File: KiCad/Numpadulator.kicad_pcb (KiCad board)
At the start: 2 copper layers, 3.4 x 3 mm, 58 parts, among them SW1 Cherry_MX_RGB_WS2812, SW10 Cherry_MX_RGB_WS2812, SW11 Cherry_MX_RGB_WS2812, SW12 Cherry_MX_RGB_WS2812, SW13 Cherry_MX_RGB_WS2812, SW14 Cherry_MX_RGB_WS2812, SW15 Cherry_MX_RGB_WS2812, SW16 Cherry_MX_RGB_WS2812, SW17 Cherry_MX_RGB_WS2812, SW18 Cherry_MX_RGB_WS2812, SW19 Rotary_Encoder_Switch, SW2 Cherry_MX_RGB_WS2812, SW3 Cherry_MX_RGB_WS2812, SW4 Cherry_MX_RGB_WS2812, SW5 Cherry_MX_RGB_WS2812, SW6 Cherry_MX_RGB_WS2812, SW7 Cherry_MX_RGB_WS2812, SW8 Cherry_MX_RGB_WS2812, SW9 Cherry_MX_RGB_WS2812, U1 PRO_MICRO_C, U2 OLED_SSD1306

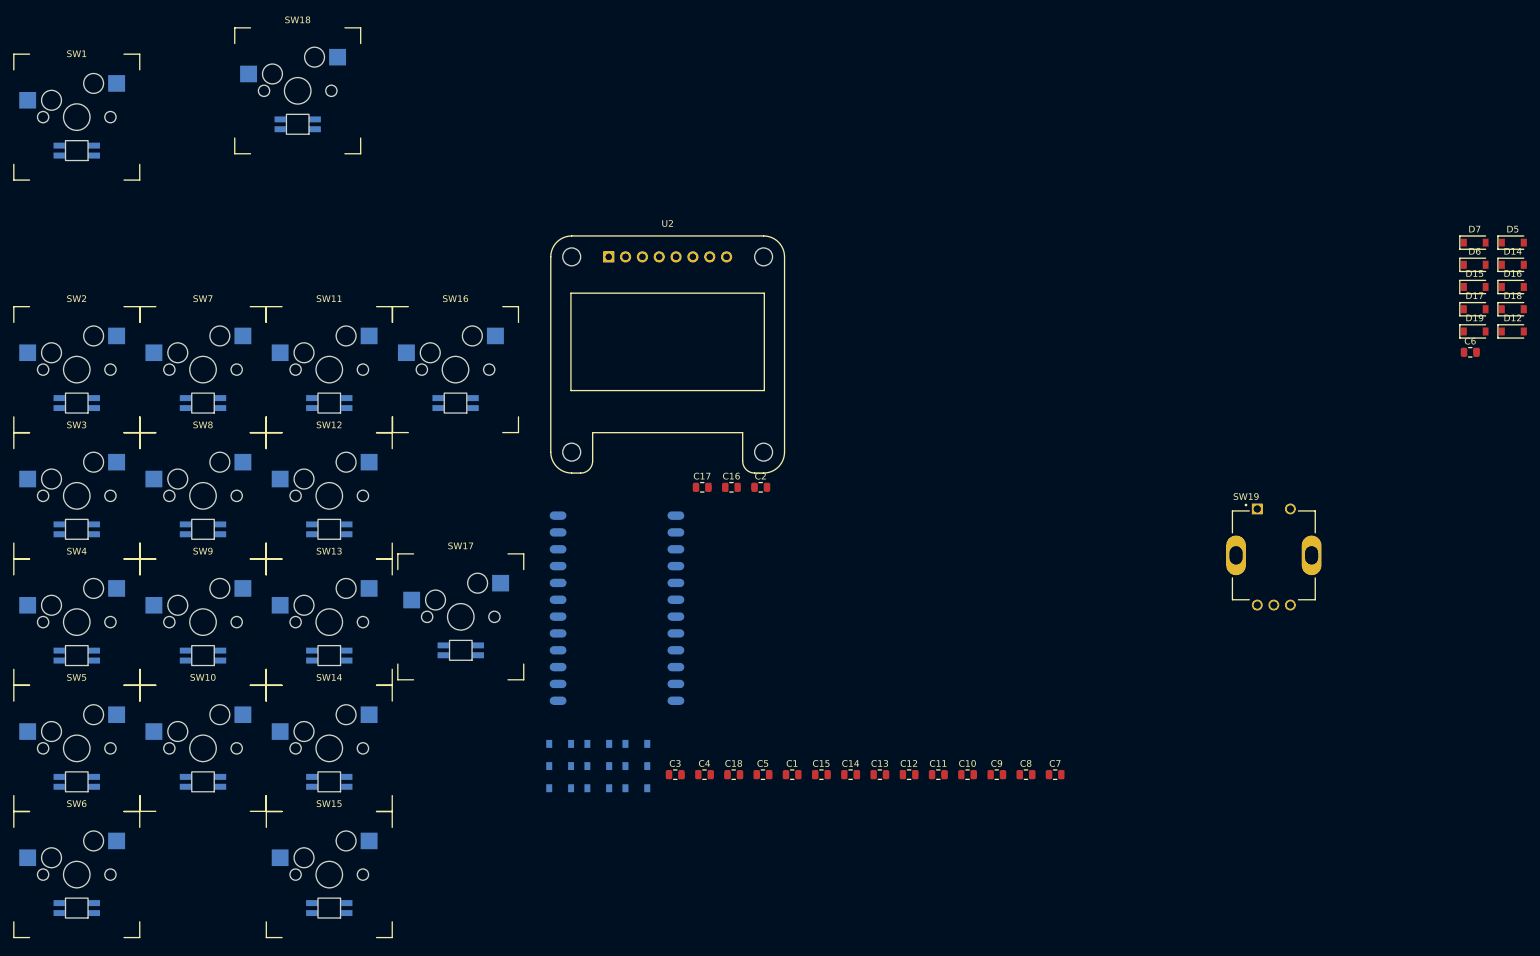
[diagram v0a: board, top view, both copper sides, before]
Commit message: More layout and frustration 3:
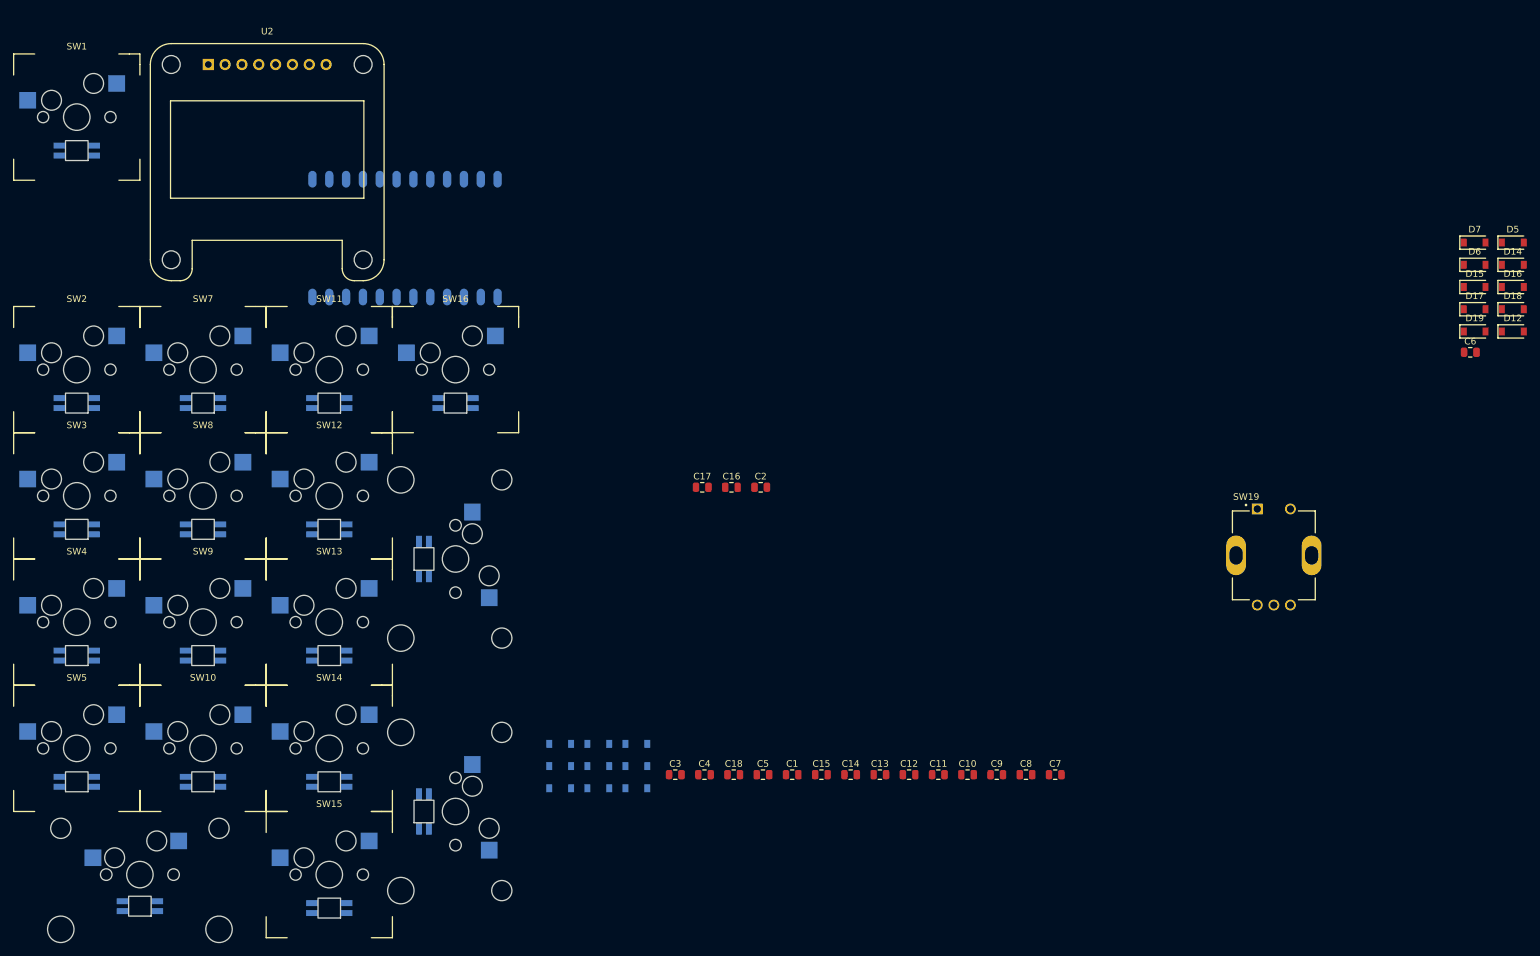
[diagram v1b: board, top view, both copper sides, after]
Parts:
- removed SW17, SW18, SW6: Cherry_MX_RGB_WS2812, Cherry MX:Cherry-MX_PCB-Mounted_LTST-A683CEGBW_Kailh_Socket
- added D20: WS2816, Custom-parts:SK6812-MINI-E, F.Cu at (73.0, 165.1)
- added D21: WS2816, Custom-parts:SK6812-MINI-E, F.Cu at (115.9, 112.7)
- added D22: WS2816, Custom-parts:SK6812-MINI-E, F.Cu at (115.9, 150.8)
- added MX1: MX-NoLED, MX_Only:MXOnly-2U-Hotswap, F.Cu at (73.0, 160.3)
- added MX2: MX-NoLED, MX_Only:MXOnly-2U-Hotswap, F.Cu at (120.7, 112.7)
- added MX3: MX-NoLED, MX_Only:MXOnly-2U-Hotswap, F.Cu at (120.7, 150.8)
- SW1, SW10, SW11, SW12, SW13, SW14, SW15, SW16, SW2, SW3, SW4, SW5, SW7, SW8, SW9: footprint Cherry MX:Cherry-MX_PCB-Mounted_LTST-A683CEGBW_Kailh_Socket -> Custom-parts:Cherry-MX_PCB-Mounted_SK6812-MINI-E_Kailh_Socket
- moved U2 67.0 mm to (83.3, 38.1)
- moved U1 62.6 mm to (114.3, 64.3), turned to 90 degrees
